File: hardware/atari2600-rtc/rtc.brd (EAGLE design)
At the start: 15 x 21.2 mm, 4 parts

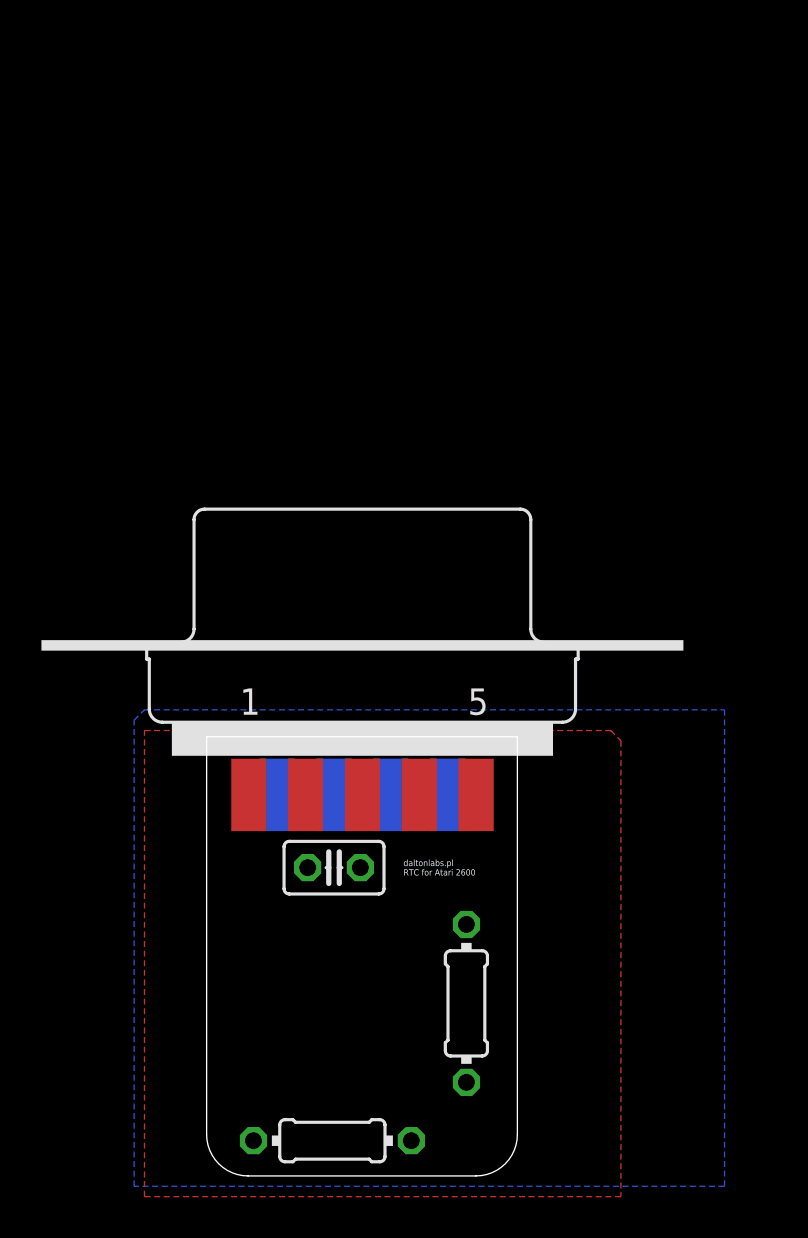
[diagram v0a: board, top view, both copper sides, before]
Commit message: Update RTC design
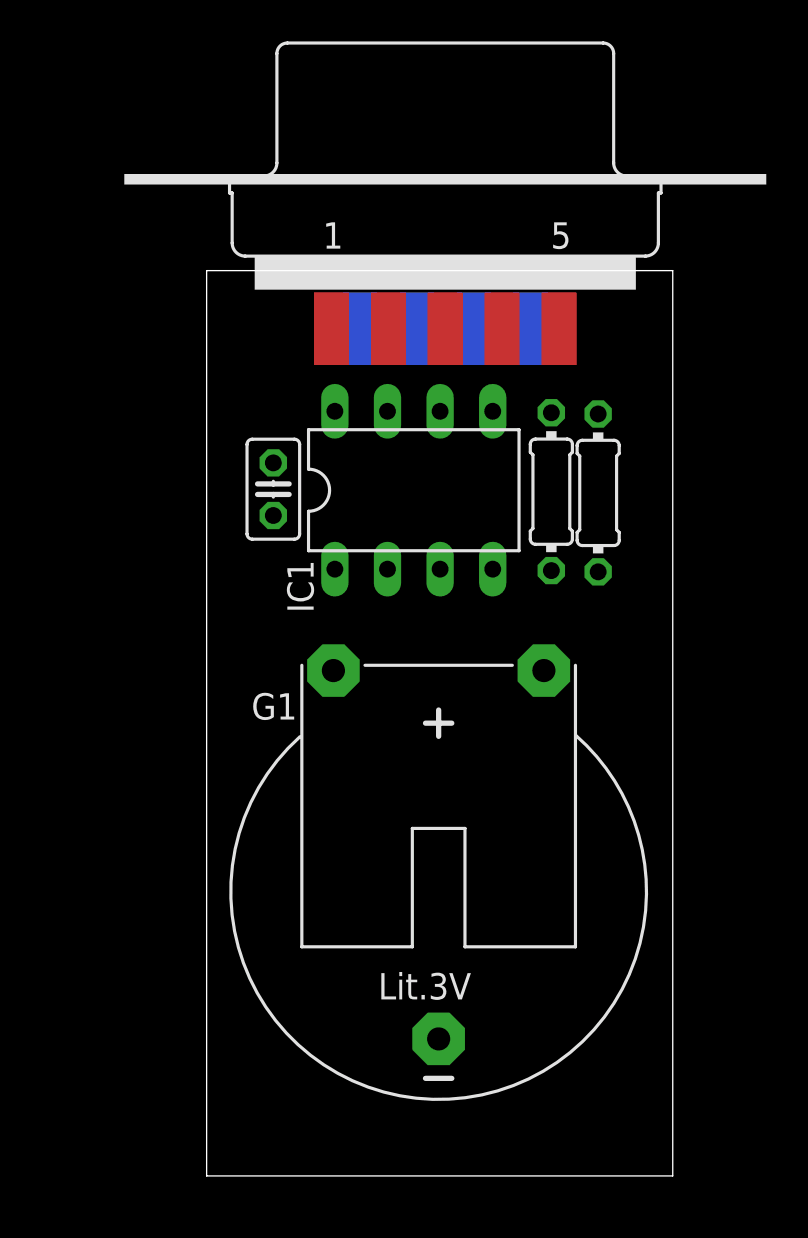
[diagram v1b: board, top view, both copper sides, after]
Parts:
- added G1: CR2032H, battery:CR2032H
- added IC1: DS1307, ic-package:DIL08
- moved R1 33.8 mm to (18.9, 33.0), turned to 270 degrees
- moved R2 25.0 mm to (16.6, 33.0)
- moved X1 22.9 mm to (11.5, 46.9)
- moved C1 18.5 mm to (3.22, 33.1), turned to 270 degrees
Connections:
- new net N$4: G1.+, IC1.3
- net GND: now also G1.-, IC1.4
- net N$1: now also IC1.5
- net N$2: now also IC1.6
- net VCC: now also IC1.8
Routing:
- removed copper zone on layer 1, net GND
- removed copper zone on layer 16, net GND
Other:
- board size 15 x 21.2 mm -> 22.5 x 43.7 mm
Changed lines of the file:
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@@
 <setting verticaltext="up"/>
 </settings>
-<grid distance="0.5" unitdist="mm" unit="mm" style="lines" multiple="1" display="yes" altdistance="5" altunitdist="mil" altunit="mil"/>
+<grid distance="0.1" unitdist="mm" unit="mm" style="lines" multiple="1" display="yes" altdistance="5" altunitdist="mil" altunit="mil"/>
 <layers>
 <layer number="1" name="Top" color="4" fill="1" visible="yes" active="yes"/>
@@
 <board>
 <plain>
-<wire x1="2" y1="0" x2="13" y2="0" width="0" layer="20"/>
-<wire x1="15" y1="2" x2="15" y2="21.2" width="0" layer="20"/>
-<wire x1="15" y1="21.2" x2="0" y2="21.2" width="0" layer="20"/>
-<wire x1="0" y1="21.2" x2="0" y2="2" width="0" layer="20"/>
-<wire x1="2" y1="0" x2="0" y2="2" width="0" layer="20" curve="-90"/>
-<wire x1="15" y1="2" x2="13" y2="0" width="0" layer="20" curve="-90"/>
-<text x="9.5" y="14.5" size="0.3048" layer="25">daltonlabs.pl
-RTC for Atari 2600</text>
-<text x="5.5" y="1" size="0.8128" layer="26" rot="MR90">daltonlabs.pl
+<wire x1="0" y1="0" x2="22.5" y2="0" width="0" layer="20"/>
+<wire x1="22.5" y1="0" x2="22.5" y2="43.7" width="0" layer="20"/>
+<wire x1="22.5" y1="43.7" x2="0" y2="43.7" width="0" layer="20"/>
+<wire x1="0" y1="43.7" x2="0" y2="0" width="0" layer="20"/>
+<text x="9.5" y="23.5" size="0.8128" layer="26" rot="MR90">daltonlabs.pl
 RTC for Atari 2600</text>
 </plain>
@@
 </autorouter>
 <elements>
-<element name="C1" library="rcl" library_urn="urn:adsk.eagle:library:334" package="C025-025X050" package3d_urn="urn:adsk.eagle:package:23629/2" value="100n" x="6.15" y="14.88" smashed="yes" rot="R180">
-<attribute name="POPULARITY" value="65" x="-26.87" y="37.74" size="1.778" layer="27" rot="R180" display="off"/>
-<attribute name="SPICEPREFIX" value="C" x="-26.87" y="37.74" size="1.778" layer="27" rot="R180" display="off"/>
-</element>
-<element name="R1" library="rcl" library_urn="urn:adsk.eagle:library:334" package="0204/7" package3d_urn="urn:adsk.eagle:package:23498/2" value="10k" x="6.07" y="1.7" smashed="yes" rot="R180">
-<attribute name="POPULARITY" value="79" x="-34.57" y="23.29" size="1.778" layer="27" rot="R180" display="off"/>
-<attribute name="SPICEPREFIX" value="R" x="-34.57" y="23.29" size="1.778" layer="27" rot="R180" display="off"/>
-</element>
-<element name="R2" library="rcl" library_urn="urn:adsk.eagle:library:334" package="0204/7" package3d_urn="urn:adsk.eagle:package:23498/2" value="10k" x="12.54" y="8.33" smashed="yes" rot="R90">
-<attribute name="POPULARITY" value="79" x="49.37" y="26.11" size="1.778" layer="27" rot="R90" display="off"/>
-<attribute name="SPICEPREFIX" value="R" x="49.37" y="26.11" size="1.778" layer="27" rot="R90" display="off"/>
-</element>
-<element name="X1" library="con-subd" library_urn="urn:adsk.eagle:library:189" package="F09D" package3d_urn="urn:adsk.eagle:package:10273/1" value="" x="7.52" y="24.44" smashed="yes">
-<attribute name="MF" value="" x="39.27" y="13.01" size="1.778" layer="27" display="off"/>
-<attribute name="MPN" value="" x="39.27" y="13.01" size="1.778" layer="27" display="off"/>
-<attribute name="OC_FARNELL" value="unknown" x="39.27" y="13.01" size="1.778" layer="27" display="off"/>
-<attribute name="OC_NEWARK" value="unknown" x="39.27" y="13.01" size="1.778" layer="27" display="off"/>
-<attribute name="POPULARITY" value="4" x="39.27" y="13.01" size="1.778" layer="27" display="off"/>
-<attribute name="VALUE" x="8.79" y="14.28" size="1.778" layer="27" ratio="10"/>
+<element name="C1" library="rcl" library_urn="urn:adsk.eagle:library:334" package="C025-025X050" package3d_urn="urn:adsk.eagle:package:23629/2" value="100n" x="3.22" y="33.15" smashed="yes" rot="R270">
+<attribute name="POPULARITY" value="65" x="-19.64" y="0.13" size="1.778" layer="27" rot="R270" display="off"/>
+<attribute name="SPICEPREFIX" value="C" x="-19.64" y="0.13" size="1.778" layer="27" rot="R270" display="off"/>
+</element>
+<element name="R1" library="rcl" library_urn="urn:adsk.eagle:library:334" package="0204/7" package3d_urn="urn:adsk.eagle:package:23498/2" value="10k" x="18.9" y="32.97" smashed="yes" rot="R270">
+<attribute name="POPULARITY" value="79" x="-2.69" y="-7.67" size="1.778" layer="27" rot="R270" display="off"/>
+<attribute name="SPICEPREFIX" value="R" x="-2.69" y="-7.67" size="1.778" layer="27" rot="R270" display="off"/>
+</element>
+<element name="R2" library="rcl" library_urn="urn:adsk.eagle:library:334" package="0204/7" package3d_urn="urn:adsk.eagle:package:23498/2" value="10k" x="16.64" y="33.03" smashed="yes" rot="R90">
+<attribute name="POPULARITY" value="79" x="53.47" y="50.81" size="1.778" layer="27" rot="R90" display="off"/>
+<attribute name="SPICEPREFIX" value="R" x="53.47" y="50.81" size="1.778" layer="27" rot="R90" display="off"/>
+</element>
+<element name="X1" library="con-subd" library_urn="urn:adsk.eagle:library:189" package="F09D" package3d_urn="urn:adsk.eagle:package:10273/1" value="" x="11.52" y="46.94" smashed="yes">
+<attribute name="MF" value="" x="43.27" y="35.51" size="1.778" layer="27" display="off"/>
+<attribute name="MPN" value="" x="43.27" y="35.51" size="1.778" layer="27" display="off"/>
+<attribute name="OC_FARNELL" value="unknown" x="43.27" y="35.51" size="1.778" layer="27" display="off"/>
+<attribute name="OC_NEWARK" value="unknown" x="43.27" y="35.51" size="1.778" layer="27" display="off"/>
+<attribute name="POPULARITY" value="4" x="43.27" y="35.51" size="1.778" layer="27" display="off"/>
+<attribute name="VALUE" x="12.79" y="36.78" size="1.778" layer="27" ratio="10"/>
+</element>
+<element name="IC1" library="ic-package" library_urn="urn:adsk.eagle:library:239" package="DIL08" package3d_urn="urn:adsk.eagle:package:29519/2" value="DS1307" x="10" y="33.1" smashed="yes">
+<attribute name="NAME" x="5.166" y="27.179" size="1.27" layer="25" ratio="10" rot="R90"/>
+<attribute name="POPULARITY" value="8" x="10" y="33.1" size="1.778" layer="27" display="off"/>
+<attribute name="VALUE" x="6.444" y="32.465" size="1.27" layer="27" ratio="10"/>
+</element>
+<element name="G1" library="battery" library_urn="urn:adsk.eagle:library:109" package="CR2032H" package3d_urn="urn:adsk.eagle:package:4585/1" value="CR2032H" x="11.2" y="13.6" smashed="yes">
+<attribute name="NAME" x="2.16" y="22.03" size="1.27" layer="25" ratio="10"/>
+<attribute name="POPULARITY" value="0" x="11.2" y="13.6" size="1.778" layer="27" display="off"/>
+<attribute name="VALUE" x="16.28" y="11.695" size="1.27" layer="27" ratio="10" rot="R90"/>
 </element>
 </elements>
@@
 <signal name="VCC">
 <contactref element="X1" pad="7"/>
-<contactref element="R2" pad="2"/>
 <contactref element="R1" pad="2"/>
 <contactref element="C1" pad="1"/>
-<wire x1="7.42" y1="14.88" x2="6.1484" y2="18.3948" width="0" layer="19" extent="16-16"/>
-<wire x1="12.54" y1="12.14" x2="7.42" y2="14.88" width="0" layer="19" extent="1-1"/>
-<wire x1="2.26" y1="1.7" x2="7.42" y2="14.88" width="0" layer="19" extent="1-1"/>
+<contactref element="R2" pad="2"/>
+<contactref element="IC1" pad="8"/>
+<wire x1="3.22" y1="34.42" x2="10.1484" y2="40.8948" width="0" layer="19" extent="16-16"/>
+<wire x1="16.64" y1="36.84" x2="3.22" y2="34.42" width="0" layer="19" extent="1-1"/>
+<wire x1="18.9" y1="29.16" x2="3.22" y2="34.42" width="0" layer="19" extent="1-1"/>
+<wire x1="6.19" y1="36.91" x2="18.9" y2="29.16" width="0" layer="19" extent="1-1"/>
 </signal>
 <signal name="GND">
 <contactref element="X1" pad="8"/>
 <contactref element="C1" pad="2"/>
-<polygon width="0" layer="1">
-<vertex x="-3" y="21.5"/>
-<vertex x="19.5" y="21.5"/>
-<vertex x="20" y="21"/>
-<vertex x="20" y="-1"/>
-<vertex x="-3" y="-1"/>
-</polygon>
-<polygon width="0" layer="16">
-<vertex x="-3.5" y="22"/>
-<vertex x="-3" y="22.5"/>
-<vertex x="25" y="22.5"/>
-<vertex x="25" y="-0.5"/>
-<vertex x="-3.5" y="-0.5"/>
-</polygon>
-<wire x1="4.88" y1="14.88" x2="8.8916" y2="18.3948" width="0" layer="19" extent="16-16"/>
+<contactref element="IC1" pad="4"/>
+<contactref element="G1" pad="-"/>
+<wire x1="3.22" y1="31.88" x2="12.8916" y2="40.8948" width="0" layer="19" extent="16-16"/>
+<wire x1="13.81" y1="29.29" x2="3.22" y2="31.88" width="0" layer="19" extent="1-1"/>
+<wire x1="11.2" y1="6.615" x2="13.81" y2="29.29" width="0" layer="19" extent="1-1"/>
 </signal>
 <signal name="N$1">
 <contactref element="X1" pad="3"/>
 <contactref element="R2" pad="1"/>
-<wire x1="12.54" y1="4.52" x2="7.52" y2="18.395" width="0" layer="19" extent="1-1"/>
+<contactref element="IC1" pad="5"/>
+<wire x1="16.64" y1="29.22" x2="11.52" y2="40.895" width="0" layer="19" extent="1-1"/>
+<wire x1="13.81" y1="36.91" x2="16.64" y2="29.22" width="0" layer="19" extent="1-1"/>
 </signal>
 <signal name="N$2">
 <contactref element="X1" pad="4"/>
 <contactref element="R1" pad="1"/>
-<wire x1="9.88" y1="1.7" x2="10.2634" y2="18.3952" width="0" layer="19" extent="1-1"/>
+<contactref element="IC1" pad="6"/>
+<wire x1="18.9" y1="36.78" x2="14.2634" y2="40.8952" width="0" layer="19" extent="1-1"/>
+<wire x1="11.27" y1="36.91" x2="18.9" y2="36.78" width="0" layer="19" extent="1-1"/>
+</signal>
+<signal name="N$4">
+<contactref element="G1" pad="+"/>
+<contactref element="IC1" pad="3"/>
+<wire x1="16.28" y1="24.395" x2="11.27" y2="29.29" width="0" layer="19" extent="1-1"/>
 </signal>
 </signals>
